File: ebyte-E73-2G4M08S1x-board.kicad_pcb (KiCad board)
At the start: 4 copper layers, 26.7 x 47 mm, 39 parts, among them J1 USB_B_Micro, J2 USB_B_Micro, J3 BAT, J4 Conn_01x18_Male, J5 Conn_01x18_Male, J6 Conn_ARM_JTAG_SWD_10, J7 Conn_02x03_Odd_Even, Q1 PMV65XP, SW1 SW_Push, U1 MCP73831-2-OT, U2 LP5907MFX-3.3, U3 CH340E, U4 E73-2G4M08S1E, U5 L3GD20, Y1 Crystal

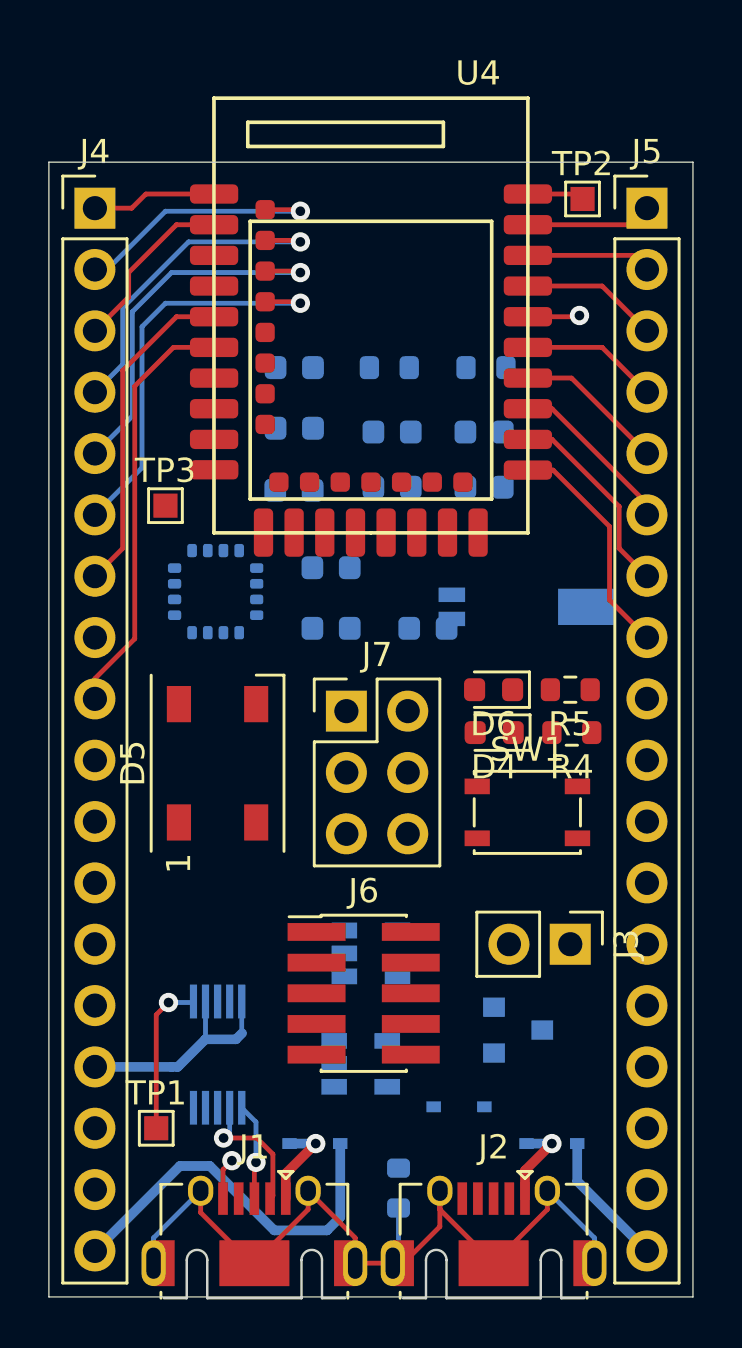
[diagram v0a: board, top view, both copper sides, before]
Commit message: Preliminary PCB layout
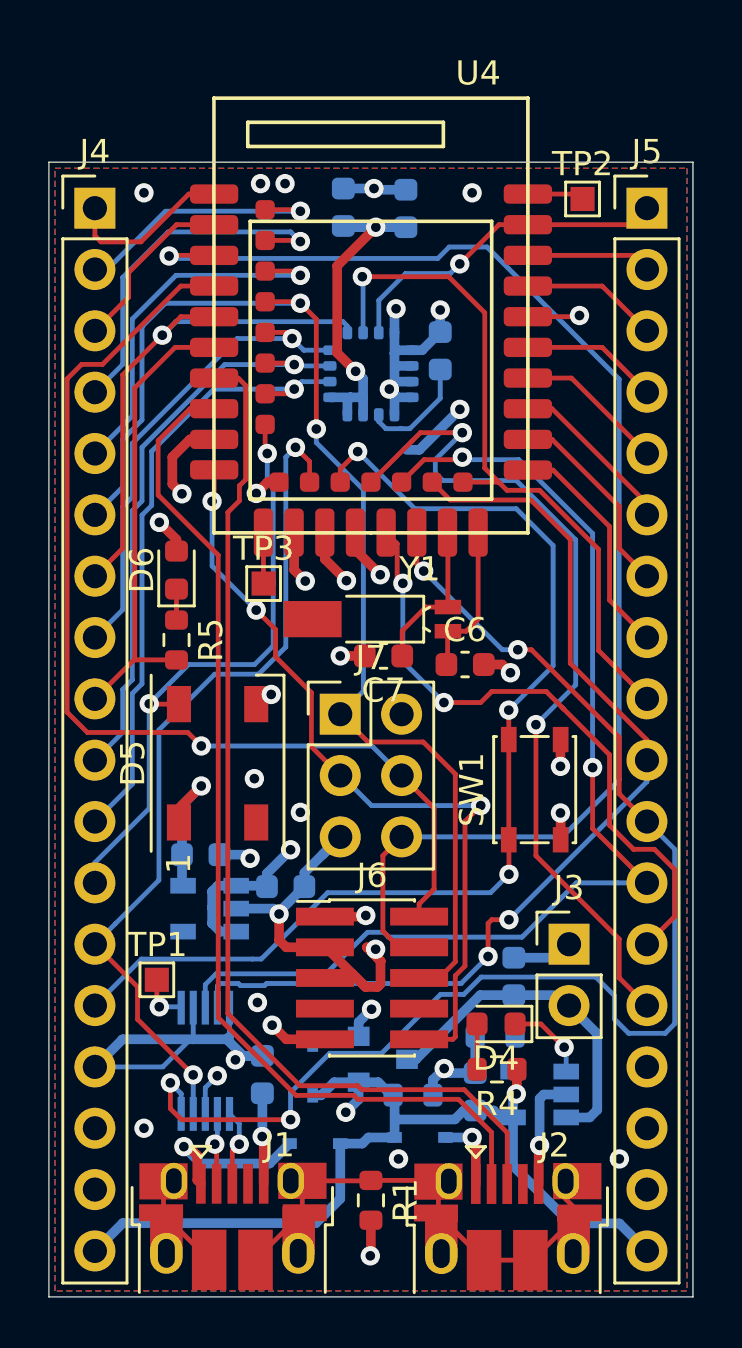
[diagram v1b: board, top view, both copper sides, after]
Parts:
- C6, C7, R1, Y1: moved to F.Cu
- J1, J2: footprint Connector_USB:USB_Micro-AB_Molex_47590-0001 -> Connector_USB:USB_Micro-B_Amphenol_10103594-0001LF_Horizontal
- moved R2 30.3 mm to (151.0, 110.1)
- moved R3 28.0 mm to (154.4, 107.7)
- moved C1 27.5 mm to (153.5, 110.0), turned to 90 degrees
- moved C3 26.8 mm to (144.7, 109.3), turned to 90 degrees
- moved C5 22.6 mm to (155.1, 105.2), turned to 90 degrees
- moved C2 21.5 mm to (145.7, 101.5)
- moved C10 17.8 mm to (148.1, 73.4), turned to 90 degrees
- moved R5 16.4 mm to (141.2, 91.3), turned to 270 degrees
- moved C4 15.6 mm to (142.2, 100.2)
- moved C9 15.2 mm to (150.7, 73.4), turned to 90 degrees
- moved R4 14.3 mm to (154.4, 109.1)
- moved D6 14.0 mm to (141.2, 88.4), turned to 90 degrees
- moved C8 12.4 mm to (152.1, 79.3), turned to 90 degrees
- moved D4 12.1 mm to (154.4, 107.2)
- moved U5 11.1 mm to (149.2, 80.3)
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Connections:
- Y1 pad 1: Net-(C6-Pad1) -> Net-(C7-Pad1)
- Y1 pad 2: Net-(C7-Pad1) -> Net-(C6-Pad1)
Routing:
- net GND: track 3.88 -> 67.2 mm, vias 2 -> 32
- net SWC: track 0.00 -> 55.6 mm, vias 0 -> 1
- net P0.05: track 0.00 -> 53.9 mm, vias 0 -> 4
- net VBUS: track 21.6 -> 71.2 mm, vias 0 -> 3
- net P0.08: track 0.00 -> 46.2 mm, vias 0 -> 2
- net P0.12: track 0.00 -> 45.0 mm, vias 0 -> 3
- net D+: track 0.00 -> 43.5 mm
- net D-: track 0.00 -> 43.2 mm
- net SWD: track 0.00 -> 43.1 mm, vias 0 -> 1
- net P0.06: track 0.00 -> 41.4 mm, vias 0 -> 2
- net P0.04: track 0.00 -> 35.6 mm, vias 0 -> 2
- net P0.07: track 0.00 -> 35.5 mm, vias 0 -> 2
- net SWO: track 16.9 -> 51.3 mm, vias 1 -> 2
- net RST: track 0.00 -> 32.8 mm, vias 0 -> 3
- net VDDH: track 0.00 -> 31.8 mm, vias 0 -> 3
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- added copper zone on B.Cu, net GND
- added copper zone on F.Cu, net GND

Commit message: Update sch, pcb, bom
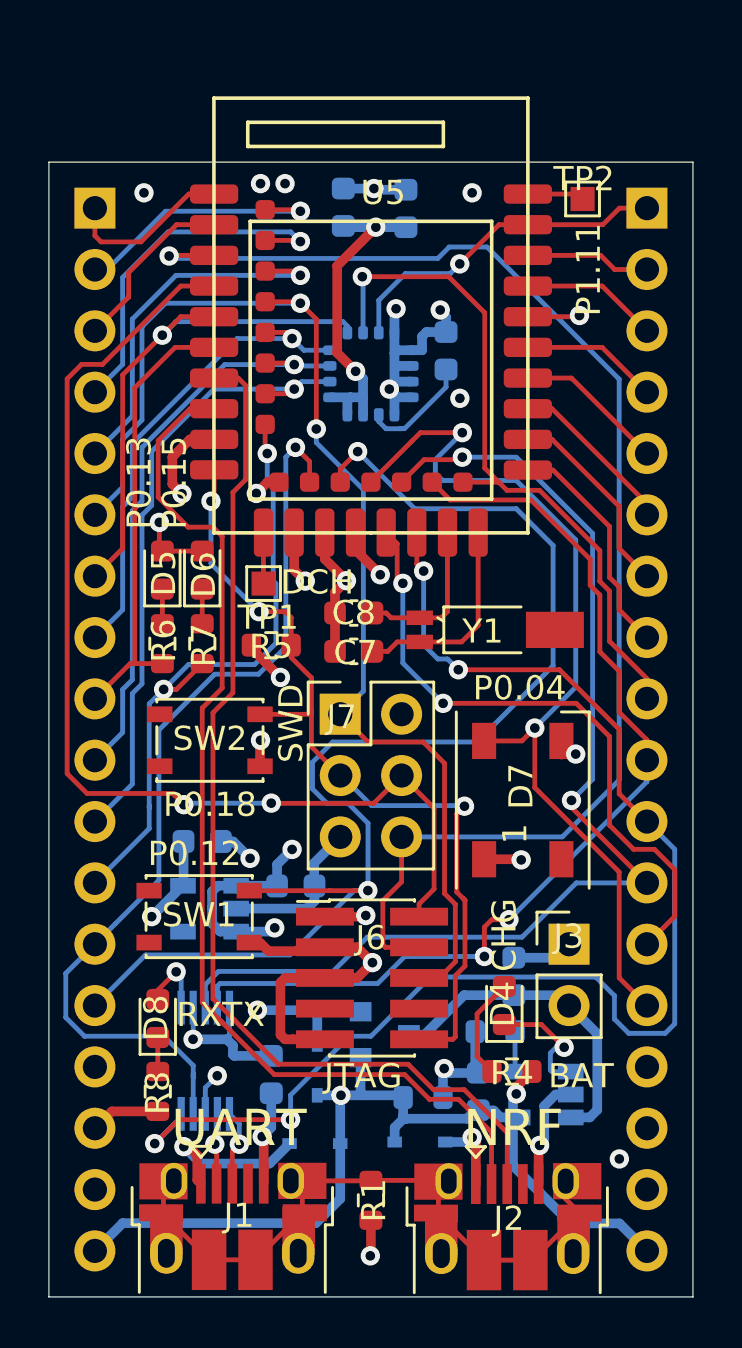
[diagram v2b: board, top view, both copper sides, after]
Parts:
- removed TP3: TestPoint, TestPoint:TestPoint_Pad_1.0x1.0mm
- removed the U5 at (149.2, 80.3)
- added D6: LED, LED_SMD:LED_0603_1608Metric, F.Cu at (142.2, 88.4)
- added D8: LED, LED_SMD:LED_0603_1608Metric, F.Cu at (140.4, 107.0)
- added R5: 10k, Resistor_SMD:R_0603_1608Metric, F.Cu at (145.1, 91.5)
- added R7: 470R, Resistor_SMD:R_0603_1608Metric, F.Cu at (142.2, 91.4)
- added R8: 470R, Resistor_SMD:R_0603_1608Metric, F.Cu at (140.4, 110.0)
- added SW2: PTS810, Button_Switch_SMD:SW_SPST_PTS810, F.Cu at (142.6, 95.4)
- added U4: L3GD20, Package_LGA:LGA-16_4x4mm_P0.65mm_LayoutBorder4x4y, B.Cu at (149.2, 80.3)
- C3: value 0.1 -> 100n
- J4, J5: moved to B.Cu
- R4: value R -> 470R
- SW1: value SW_Push -> PTS810
- Y1: value Crystal -> 32768
- moved TP1 17.0 mm to (144.8, 89.0)
- moved SW1 14.9 mm to (142.1, 102.7), turned to 0 degrees
- moved D7 12.7 mm to (155.5, 97.9)
- moved Y1 5.10 mm to (154.4, 90.9), turned to 90 degrees
- moved C7 4.64 mm to (148.5, 91.8), turned to 180 degrees
- moved C8 2.16 mm to (148.5, 90.2)
- moved Q1 1.02 mm to (149.8, 107.6)
- moved D4 0.84 mm to (154.7, 106.4), turned to 90 degrees
- moved R4 0.63 mm to (155.1, 109.2)
- moved R6 0.60 mm to (140.6, 91.4)
- moved D5 0.58 mm to (140.6, 88.4)
- moved C4 0.55 mm to (142.2, 99.6)
- moved R2 0.43 mm to (151.4, 110.2)
- moved C2 0.42 mm to (146.1, 101.5)
- moved C3 0.37 mm to (145.1, 109.3)
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- renumbered C8 to C6, C6 to C7, C7 to C8, D6 to D5, D5 to D7, R5 to R6, U4 to U5
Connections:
- C7 pad 1: Net-(C6-Pad1) (its old number) -> Net-(C7-Pad1)
- C8 pad 1: Net-(C7-Pad1) -> Net-(C8-Pad1)
- D7 pad 4: P0.15 -> P0.04
- U3 pad 6: Net-(TP1-Pad1) -> Net-(D8-Pad2)
- U5 pad 11: Net-(C6-Pad1) (its old number) -> Net-(C7-Pad1)
- U5 pad 13: Net-(C7-Pad1) -> Net-(C8-Pad1)
- U5 pad 25: Net-(TP3-Pad1) -> Net-(TP1-Pad1)
- Y1 pad 2: Net-(C6-Pad1) (its old number) -> Net-(C8-Pad1)
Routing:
- net VDD: track 41.5 -> 33.5 mm, vias 7 -> 9
- net P0.12: track 45.0 -> 52.4 mm, vias 3 -> 2
- net Net-(C8-Pad1): track 0.00 -> 6.57 mm
- net Net-(C6-Pad1) (its old number): track 6.08 -> 0.00 mm
- net P0.07: track 35.5 -> 38.6 mm, vias 2 -> 1
- net Net-(D8-Pad2): track 0.00 -> 3.08 mm, vias 0 -> 1
- net SWD: track 43.1 -> 45.7 mm, vias 1 -> 2
- net Net-(D4-Pad2): track 1.88 -> 4.24 mm
- net P0.04: track 35.6 -> 38.0 mm
- net RST: track 32.8 -> 35.0 mm
- net Net-(C7-Pad1): track 6.43 -> 8.66 mm
- net Net-(TP3-Pad1): track 2.11 -> 0.00 mm
- net P0.05: track 53.9 -> 55.8 mm
- net Net-(J1-Pad6): track 25.6 -> 27.5 mm
- net Net-(D4-Pad1): track 3.47 -> 5.23 mm
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- removed copper zone on B.Cu, net GND
- removed copper zone on F.Cu, net GND
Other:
- board text added: "BAT"
- board text added: "CHG"
- board text added: "DCH"
- board text added: "JTAG"
- board text added: "NRF"
- board text added: "P0.04"
- board text added: "P0.12"
- board text added: "P0.13"
- board text added: "P0.15"
- board text added: "P0.18"
- board text added: "P1.11"
- board text added: "RXTX"
- board text added: "SWD"
- board text added: "UART"
